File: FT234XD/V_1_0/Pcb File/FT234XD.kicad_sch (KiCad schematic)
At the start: 11 parts, among them J2 USB_A, Q2 AO3401A, U1 FT234XD, U3 USBLC6-2SC6

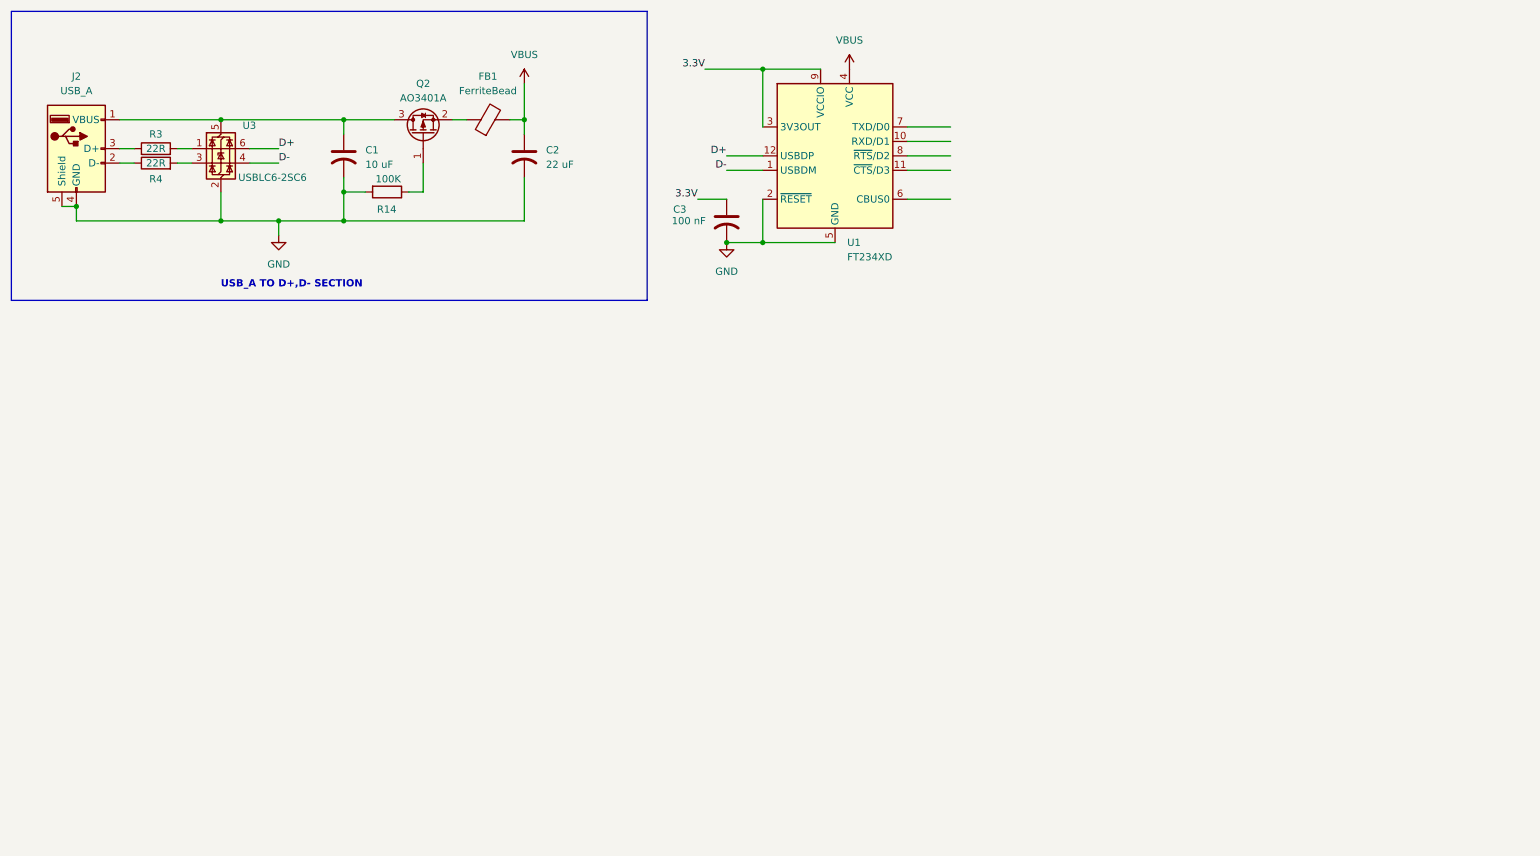
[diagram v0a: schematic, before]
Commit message: Some update
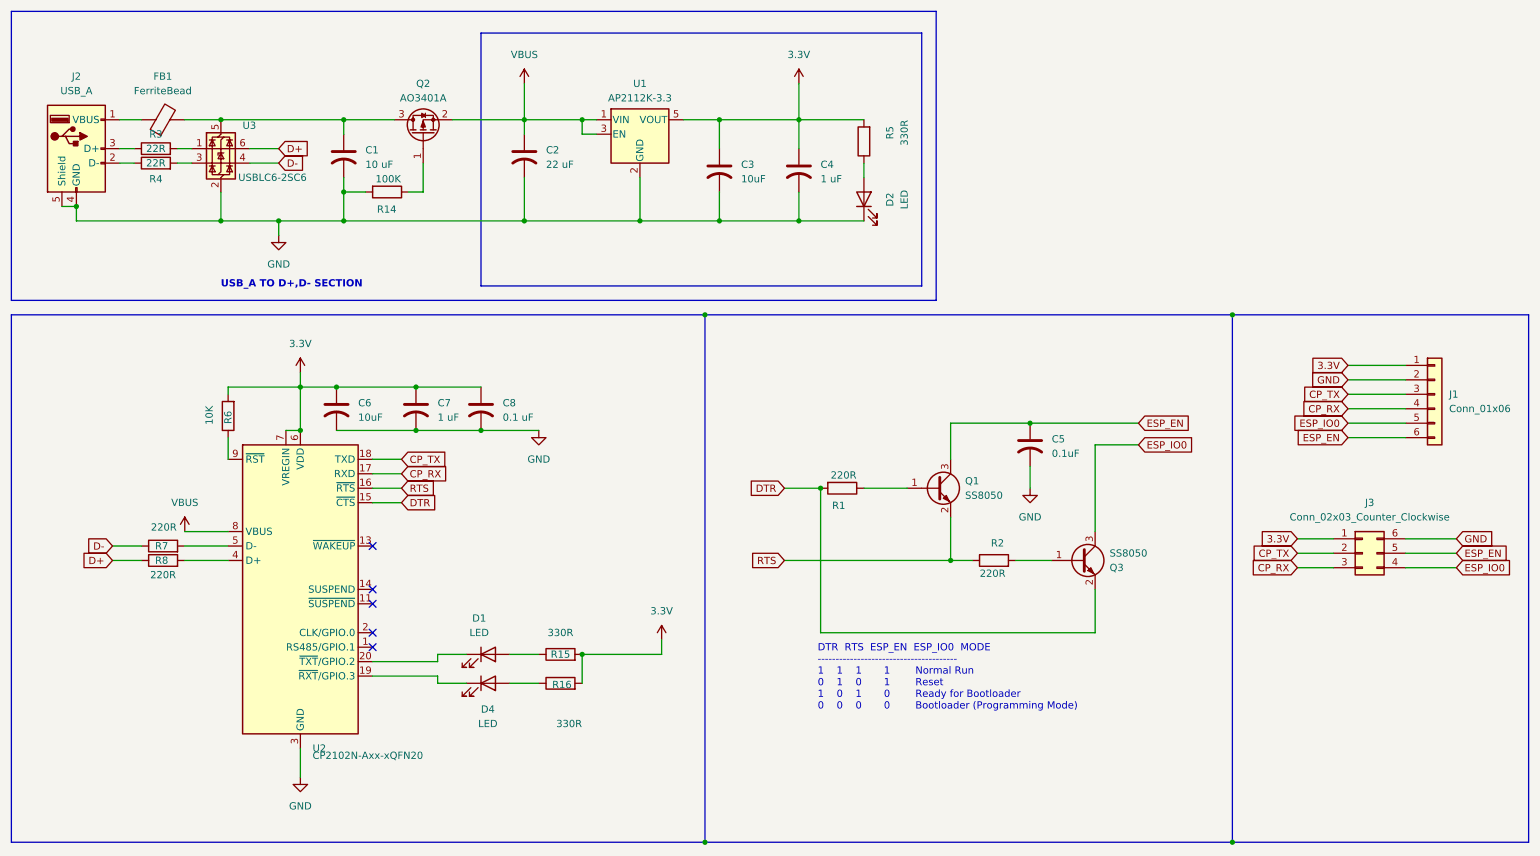
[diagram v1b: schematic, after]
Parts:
- removed U1: FT234XD, Package_DFN_QFN:WDFN-12-1EP_3x3mm_P0.45mm_EP1.7x2.5mm, symbol Interface_USB:FT234XD
- added C4, C7: 1 uF, Capacitor_SMD:C_0805_2012Metric_Pad1.18x1.45mm_HandSolder, symbol Device:C_US
- added C5: 0.1uF, Capacitor_SMD:C_0805_2012Metric_Pad1.18x1.45mm_HandSolder, symbol Device:C_US
- added C6: 10uF, Capacitor_SMD:C_0805_2012Metric_Pad1.18x1.45mm_HandSolder, symbol Device:C_US
- added C8: 0.1 uF, Capacitor_SMD:C_0805_2012Metric_Pad1.18x1.45mm_HandSolder, symbol Device:C_US
- added D1, D2, D4: LED, LED_SMD:LED_0805_2012Metric_Pad1.15x1.40mm_HandSolder, symbol Device:LED
- added J1: Conn_01x06, Connector_PinSocket_2.54mm:PinSocket_1x06_P2.54mm_Vertical, symbol Connector_Generic:Conn_01x06
- added J3: Conn_02x03_Counter_Clockwise, Connector_PinSocket_2.54mm:PinSocket_2x03_P2.54mm_Vertical_SMD, symbol Connector_Generic:Conn_02x03_Counter_Clockwise
- added Q1, Q3: SS8050, Package_TO_SOT_SMD:SOT-23, symbol Transistor_BJT:SS8050
- added R1, R2, R7, R8: 220R, Resistor_SMD:R_0805_2012Metric_Pad1.20x1.40mm_HandSolder, symbol Device:R
- added R15, R16, R5: 330R, Resistor_SMD:R_0805_2012Metric_Pad1.20x1.40mm_HandSolder, symbol Device:R
- added R6: 10K, Resistor_SMD:R_0805_2012Metric_Pad1.20x1.40mm_HandSolder, symbol Device:R
- added U1: AP2112K-3.3, Package_TO_SOT_SMD:SOT-23-5, symbol Regulator_Linear:AP2112K-3.3
- added U2: CP2102N-Axx-xQFN20, Package_DFN_QFN:SiliconLabs_QFN-20-1EP_3x3mm_P0.5mm_EP1.8x1.8mm, symbol Interface_USB:CP2102N-Axx-xQFN20
- C3: value 100 nF -> 10uF
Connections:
- net 3.3V: now also C4.1, C6.1, C7.1, C8.1, J1.1 (Pin_1), J3.1 (Pin_1), R15.2, R16.2, R5.2, R6.2, U1.5 (VOUT), U2.6 (VDD), U2.7 (VREGIN)
- net D+: now also R8.1
- net D-: now also R7.1
- net GND: now also C4.2, C5.2, C6.2, C7.2, C8.2, D2.1 (K), J1.2 (Pin_2), J3.6 (Pin_6), U1.2 (GND), U2.12 (GND), U2.21 (GND), U2.3 (GND)
- net VBUS: now also Q2.2 (S), U1.1 (VIN), U1.3 (EN), U2.8 (VBUS); no longer FB1.2
- net at C1.1, Q2.3 (D), U3.5 (VBUS): now also FB1.2; no longer J2.1 (VBUS)
- net at FB1.1: now also J2.1 (VBUS); no longer Q2.2 (S)
- new net: Q1.1 (B), R1.1
- new net: D1.2 (A), R15.1
- new net: D2.2 (A), R5.1
- new net: D4.2 (A), R16.1
- new net: R6.1, U2.9 (~{RST})
- new net: R7.2, U2.5 (D-)
- new net: Q3.1 (B), R2.2
- new net: D4.1 (K), U2.19 (~{RXT}/GPIO.3)
- new net: D1.1 (K), U2.20 (~{TXT}/GPIO.2)
- new net: R8.2, U2.4 (D+)
- new net CP_RX: J1.4 (Pin_4), J3.3 (Pin_3), U2.17 (RXD)
- new net CP_TX: J1.3 (Pin_3), J3.2 (Pin_2), U2.18 (TXD)
- new net DTR: Q3.2 (E), R1.2, U2.15 (~{CTS})
- new net ESP_EN: C5.1, J1.6 (Pin_6), J3.5 (Pin_5), Q1.3 (C)
- new net ESP_IO0: J1.5 (Pin_5), J3.4 (Pin_4), Q3.3 (C)
- new net RTS: Q1.2 (E), R2.1, U2.16 (~{RTS})
- no-connect marks 0 -> 5
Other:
- note added: "DTR RTS ESP_EN ESP_IO0 MODE --------------------------------------- 1 1 1 1 Normal Run 0 1 0 1 Reset 1 0 1 0 Ready for Bootloader 0 0 0 0 Bootloader (Programming Mode)"
- moved on the sheet: FB1
